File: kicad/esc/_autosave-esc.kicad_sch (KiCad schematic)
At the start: 107 parts, among them J2 Motor, Q1 IRF540N, Q2 IRF540N, Q3 IRF540N, Q4 IRF540N, Q5 IRF540N, Q6 IRF540N, Q7 2N3904, U1 IR2110, U10 4N35, U11 4N35, U12 4N35, U13 4N35, U14 4N35, U15 4N35, U2 IR2110, U3 IR2110, U4 LM393, U5 LM393, U6 LM7805_TO220, U7 4N35, U8 4N35, U9 4N35

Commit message: RC1
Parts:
- R26, R27, R29, R30, R33, R34: footprint Resistor_THT:R_Axial_DIN0204_L3.6mm_D1.6mm_P2.54mm_Vertical -> Resistor_THT:R_Axial_DIN0207_L6.3mm_D2.5mm_P7.62mm_Horizontal
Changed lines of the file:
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@@
 			)
 		)
-		(property "Footprint" "Resistor_THT:R_Axial_DIN0204_L3.6mm_D1.6mm_P2.54mm_Vertical"
+		(property "Footprint" "Resistor_THT:R_Axial_DIN0207_L6.3mm_D2.5mm_P7.62mm_Horizontal"
 			(at 25.4 102.108 90)
 			(effects
@@
 			)
 		)
-		(property "Footprint" "Resistor_THT:R_Axial_DIN0204_L3.6mm_D1.6mm_P2.54mm_Vertical"
+		(property "Footprint" "Resistor_THT:R_Axial_DIN0207_L6.3mm_D2.5mm_P7.62mm_Horizontal"
 			(at 25.4 32.258 90)
 			(effects
@@
 			)
 		)
-		(property "Footprint" "Resistor_THT:R_Axial_DIN0204_L3.6mm_D1.6mm_P2.54mm_Vertical"
+		(property "Footprint" "Resistor_THT:R_Axial_DIN0207_L6.3mm_D2.5mm_P7.62mm_Horizontal"
 			(at 25.4 135.128 90)
 			(effects
@@
 			)
 		)
-		(property "Footprint" "Resistor_THT:R_Axial_DIN0204_L3.6mm_D1.6mm_P2.54mm_Vertical"
+		(property "Footprint" "Resistor_THT:R_Axial_DIN0207_L6.3mm_D2.5mm_P7.62mm_Horizontal"
 			(at 25.4 84.328 90)
 			(effects
@@
 			)
 		)
-		(property "Footprint" "Resistor_THT:R_Axial_DIN0204_L3.6mm_D1.6mm_P2.54mm_Vertical"
+		(property "Footprint" "Resistor_THT:R_Axial_DIN0207_L6.3mm_D2.5mm_P7.62mm_Horizontal"
 			(at 25.4 50.038 90)
 			(effects
@@
 			)
 		)
-		(property "Footprint" "Resistor_THT:R_Axial_DIN0204_L3.6mm_D1.6mm_P2.54mm_Vertical"
+		(property "Footprint" "Resistor_THT:R_Axial_DIN0207_L6.3mm_D2.5mm_P7.62mm_Horizontal"
 			(at 25.4 152.908 90)
 			(effects

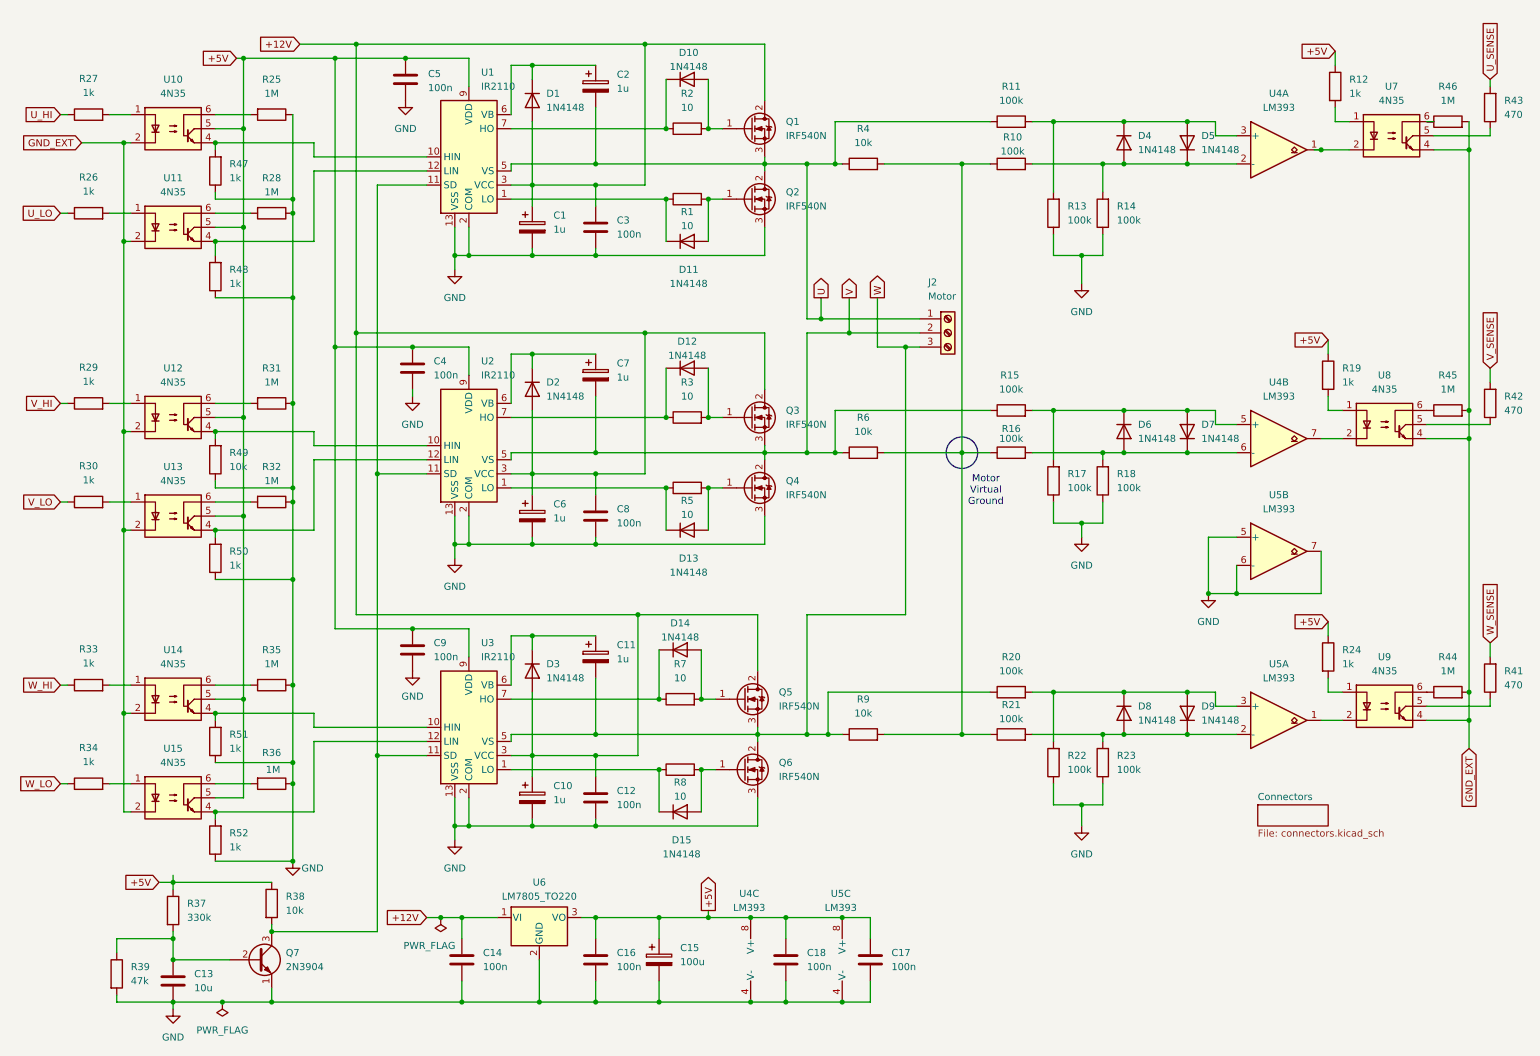
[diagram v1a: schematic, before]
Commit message: WIP
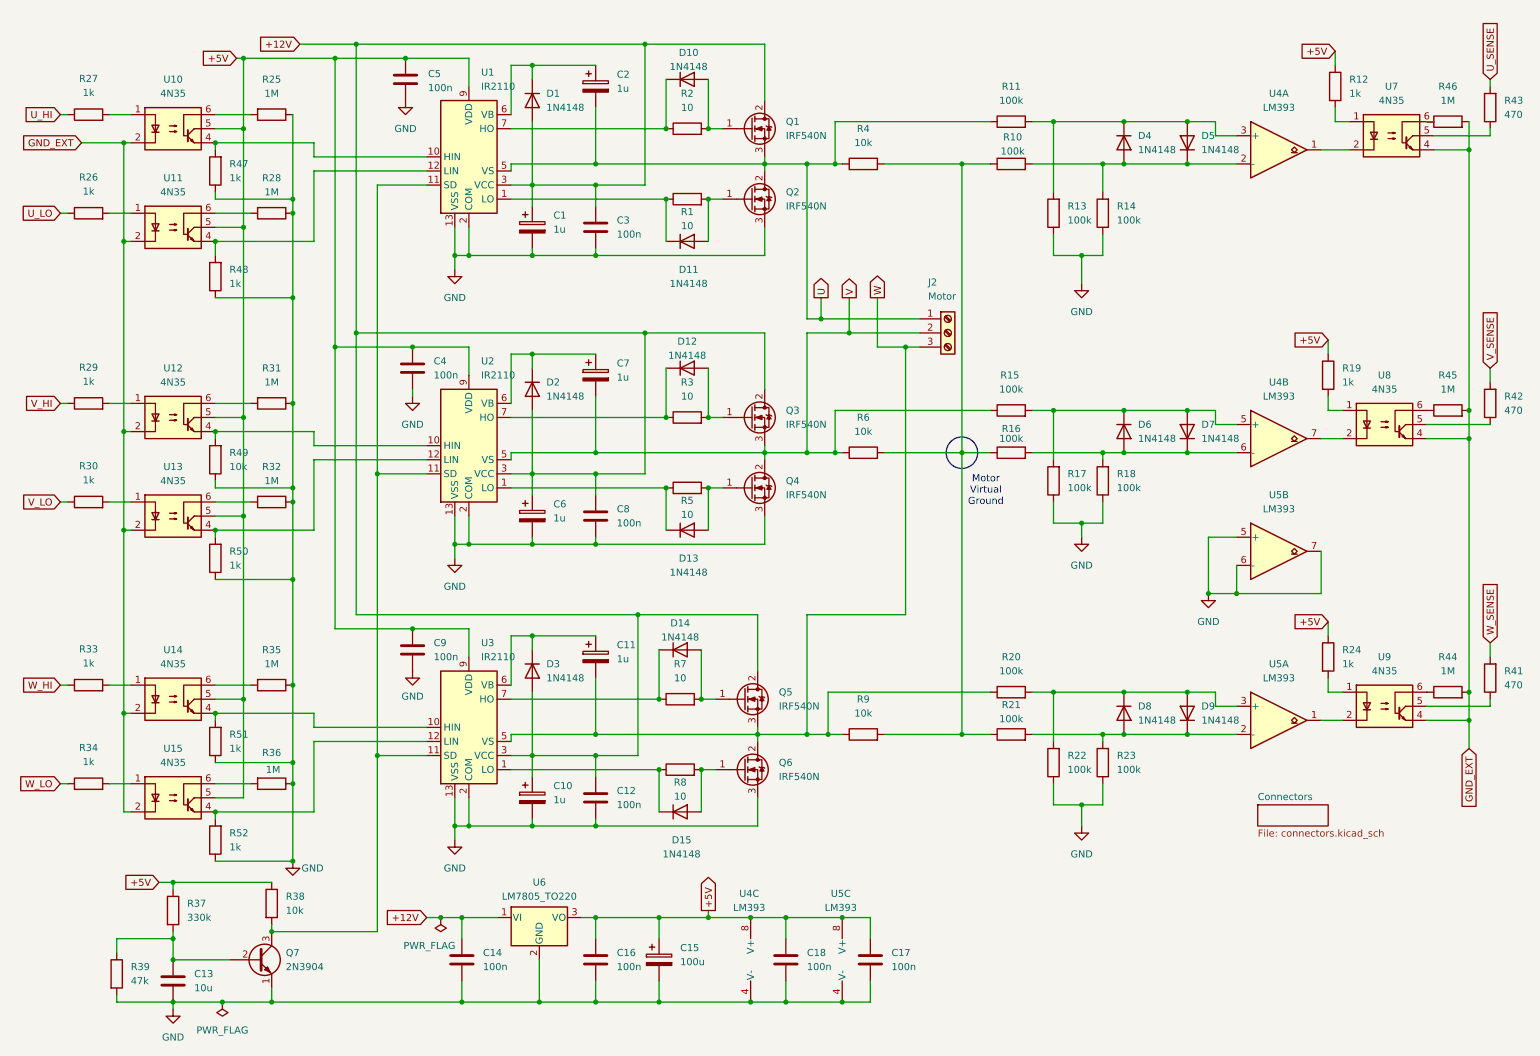
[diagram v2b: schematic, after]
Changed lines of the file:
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@@
 	)
 	(junction
-		(at 247.65 36.83)
-		(diameter 0)
-		(color 0 0 0 0)
-	)
-	(junction
 		(at 125.73 17.78)
 		(diameter 0)
@@
 	(wire
 		(pts
-			(xy 247.65 36.83) (xy 252.73 36.83)
-		)
-		(stroke
-			(width 0)
-			(type default)
-		)
-	)
-	(wire
-		(pts
 			(xy 278.13 125.73) (xy 278.13 128.27)
 		)
@@
 	(wire
 		(pts
-			(xy 246.38 36.83) (xy 247.65 36.83)
-		)
-		(stroke
-			(width 0)
-			(type default)
-		)
-	)
-	(wire
-		(pts
 			(xy 93.98 123.19) (xy 93.98 128.27)
 		)
@@
 	(wire
 		(pts
+			(xy 247.65 36.83) (xy 252.73 36.83)
+		)
+		(stroke
+			(width 0)
+			(type default)
+		)
+	)
+	(wire
+		(pts
 			(xy 154.94 120.65) (xy 154.94 142.24)
 		)
@@
 		)
 		(stroke
-			(width 0)
-			(type default)
-		)
-	)
-	(wire
-		(pts
-			(xy 40.64 167.64) (xy 40.64 168.91)
-		)
-		(stroke
